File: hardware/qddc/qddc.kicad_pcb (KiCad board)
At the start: 2 copper layers, 37 parts, among them IC1 FST3253MTCX, IC2 OPA2350UA, J1 In_cos, J2 In_sin, J3 In_RF, J4 PWR, J5 Out_I, J6 Out_Q, T1 ETC4-1-2TR

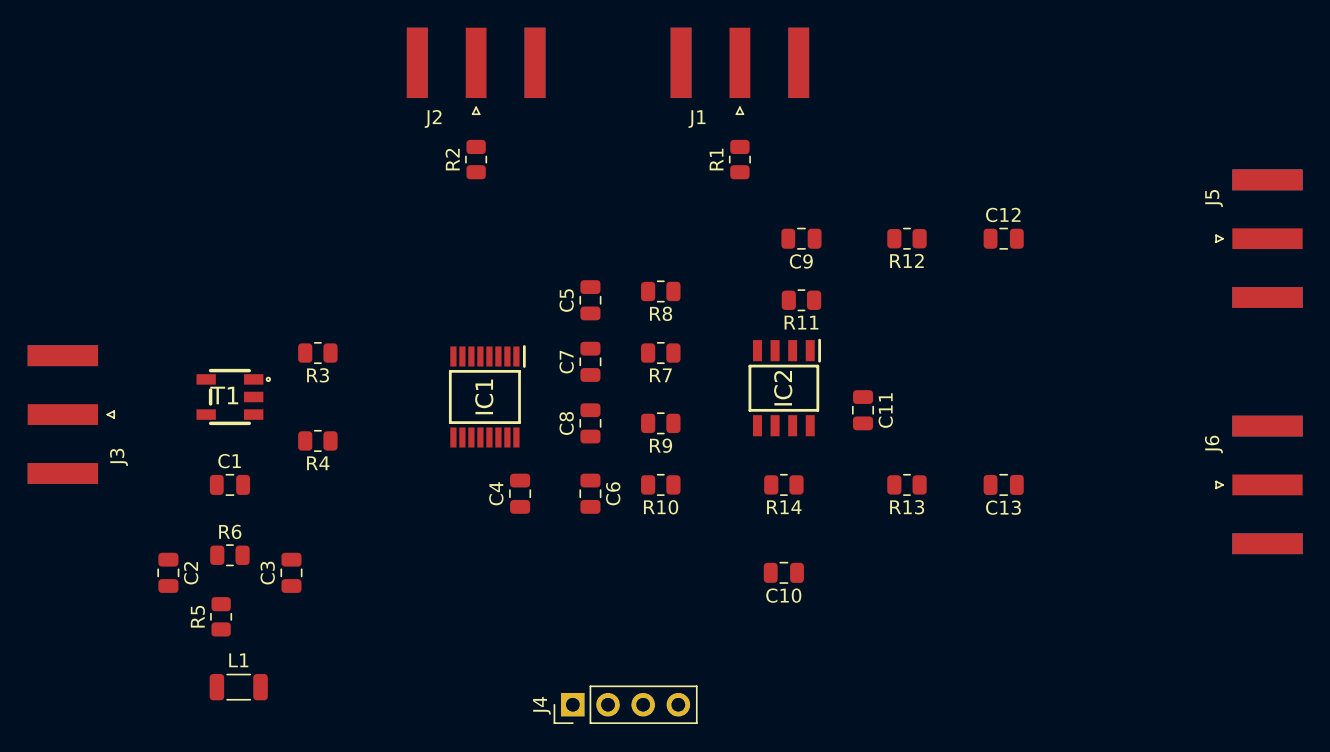
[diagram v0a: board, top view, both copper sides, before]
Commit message: PCB for Quad DDC
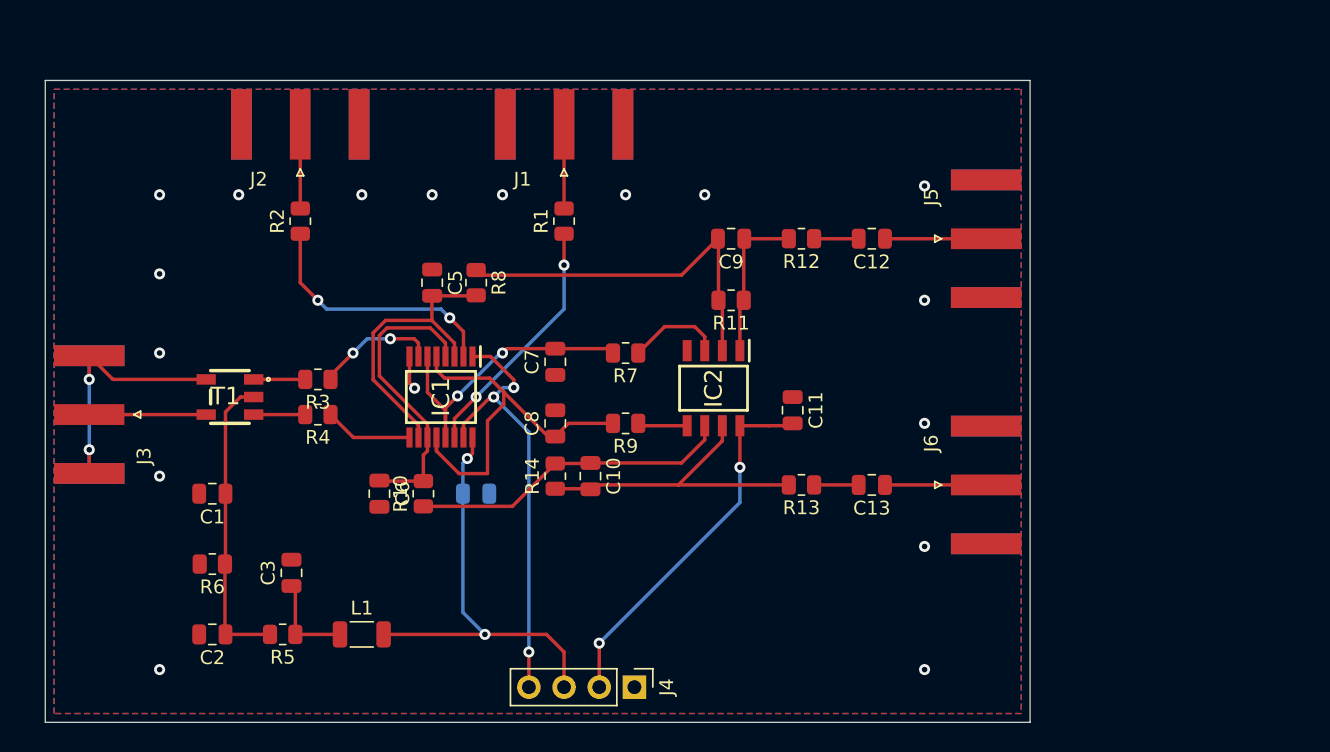
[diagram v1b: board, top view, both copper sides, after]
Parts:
- C4: moved to B.Cu
- moved J5 20.3 mm to (164.5, 94.6)
- moved J6 20.3 mm to (164.5, 112.4)
- moved R10 17.2 mm to (123.8, 113.0), turned to 90 degrees
- moved R14 16.5 mm to (133.3, 111.8), turned to 90 degrees
- moved C10 15.6 mm to (135.9, 111.8), turned to 270 degrees
- moved C6 15.2 mm to (120.7, 113.0)
- moved J2 13.5 mm to (114.9, 86.4)
- moved R2 13.5 mm to (114.9, 93.3)
- moved J1 13.5 mm to (134.0, 86.4)
- moved R1 13.5 mm to (134.0, 93.3)
- moved R8 13.4 mm to (127.6, 97.8), turned to 270 degrees
- moved C5 11.5 mm to (124.5, 97.8), turned to 270 degrees
- moved L1 9.67 mm to (119.4, 123.2)
- moved C12 9.53 mm to (156.2, 94.6), turned to 180 degrees
- moved C13 9.53 mm to (156.2, 112.4)
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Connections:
- IC2 pad 6: Net-(C10-Pad2) -> Net-(C10-Pad1)
- IC2 pad 7: Net-(C10-Pad1) -> Net-(C10-Pad2)
- J4 pad 1: PTT -> GND
- J4 pad 4: GND -> PTT
- R10 pad 1: Net-(C10-Pad2) -> Net-(C10-Pad1)
- R13 pad 2: Net-(C10-Pad1) -> Net-(C10-Pad2)
- R14 pad 1: Net-(C10-Pad1) -> Net-(C10-Pad2)
- R14 pad 2: Net-(C10-Pad2) -> Net-(C10-Pad1)
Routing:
- net PTT: track 0.00 -> 32.0 mm, vias 0 -> 3
- net VCC: track 0.00 -> 31.3 mm, vias 0 -> 2
- net Net-(C8-Pad1): track 0.00 -> 28.7 mm
- net VAA: track 0.00 -> 27.0 mm, vias 0 -> 2
- net Net-(C9-Pad2): track 0.00 -> 26.9 mm
- net Net-(C10-Pad1): track 0.00 -> 23.7 mm
- net Net-(C10-Pad2): track 0.00 -> 23.0 mm
- net Net-(C5-Pad2): track 0.00 -> 21.8 mm
- net Net-(C1-Pad1): track 0.00 -> 21.8 mm
- net Net-(C6-Pad1): track 0.00 -> 21.7 mm
- net Net-(C7-Pad2): track 0.00 -> 21.3 mm, vias 0 -> 2
- net Net-(J3-Pad2): track 0.00 -> 21.1 mm, vias 0 -> 2
- net Net-(IC1-Pad2): track 0.00 -> 18.6 mm, vias 0 -> 2
- net Net-(IC1-Pad14): track 0.00 -> 18.0 mm, vias 0 -> 2
- net Net-(C9-Pad1): track 0.00 -> 11.4 mm
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- added copper zone on B.Cu, net GND
- added copper zone on F.Cu, net GND
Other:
- board outline added: 71.1 x 46.4 mm
